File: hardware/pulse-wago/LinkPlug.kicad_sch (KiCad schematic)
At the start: 4 parts, among them J1901 2x05_Horizontal, U1901 THVD24x2

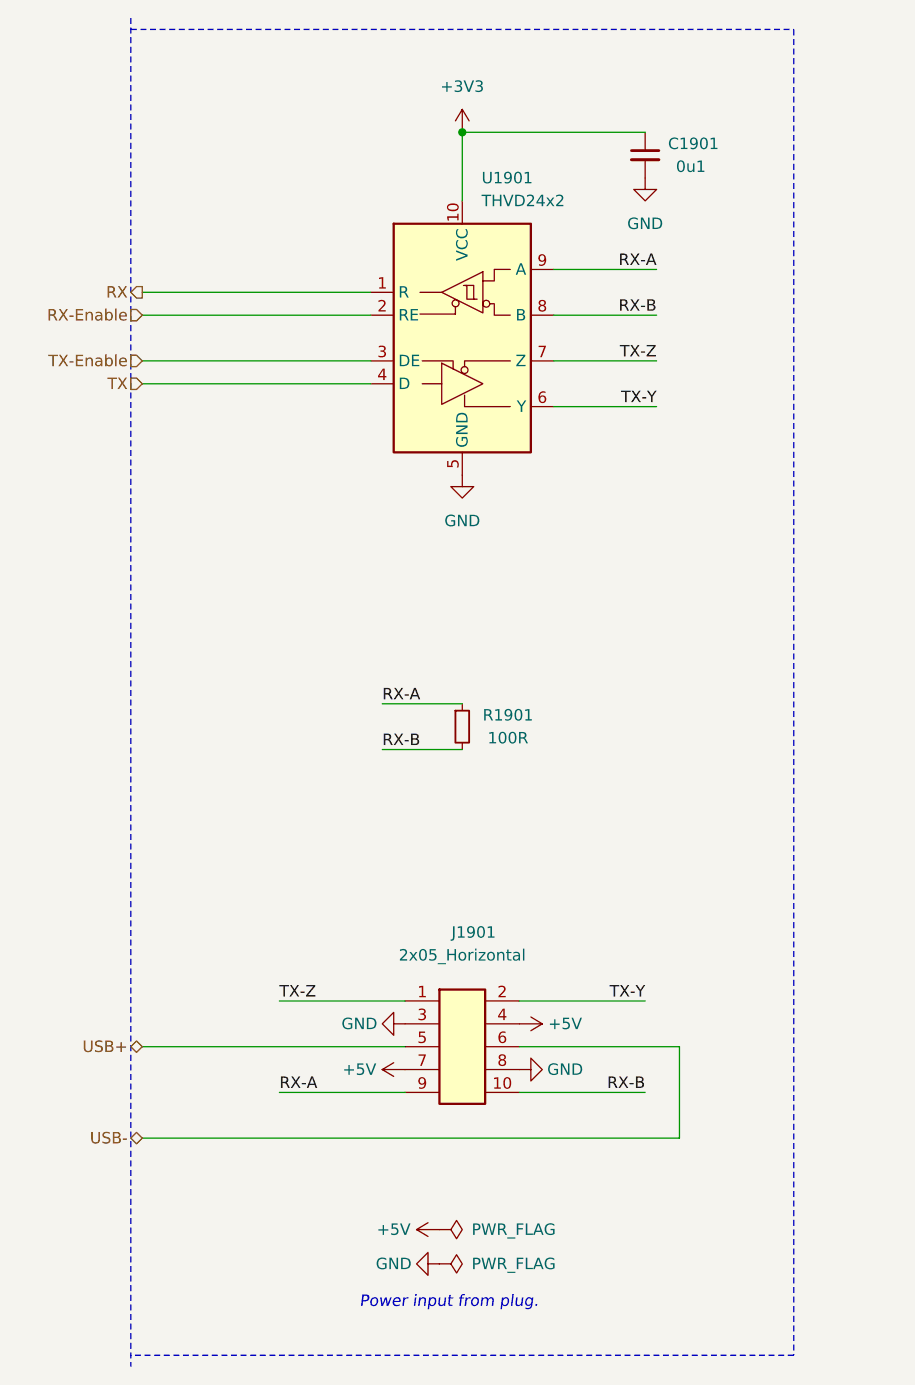
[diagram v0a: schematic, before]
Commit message: Update library
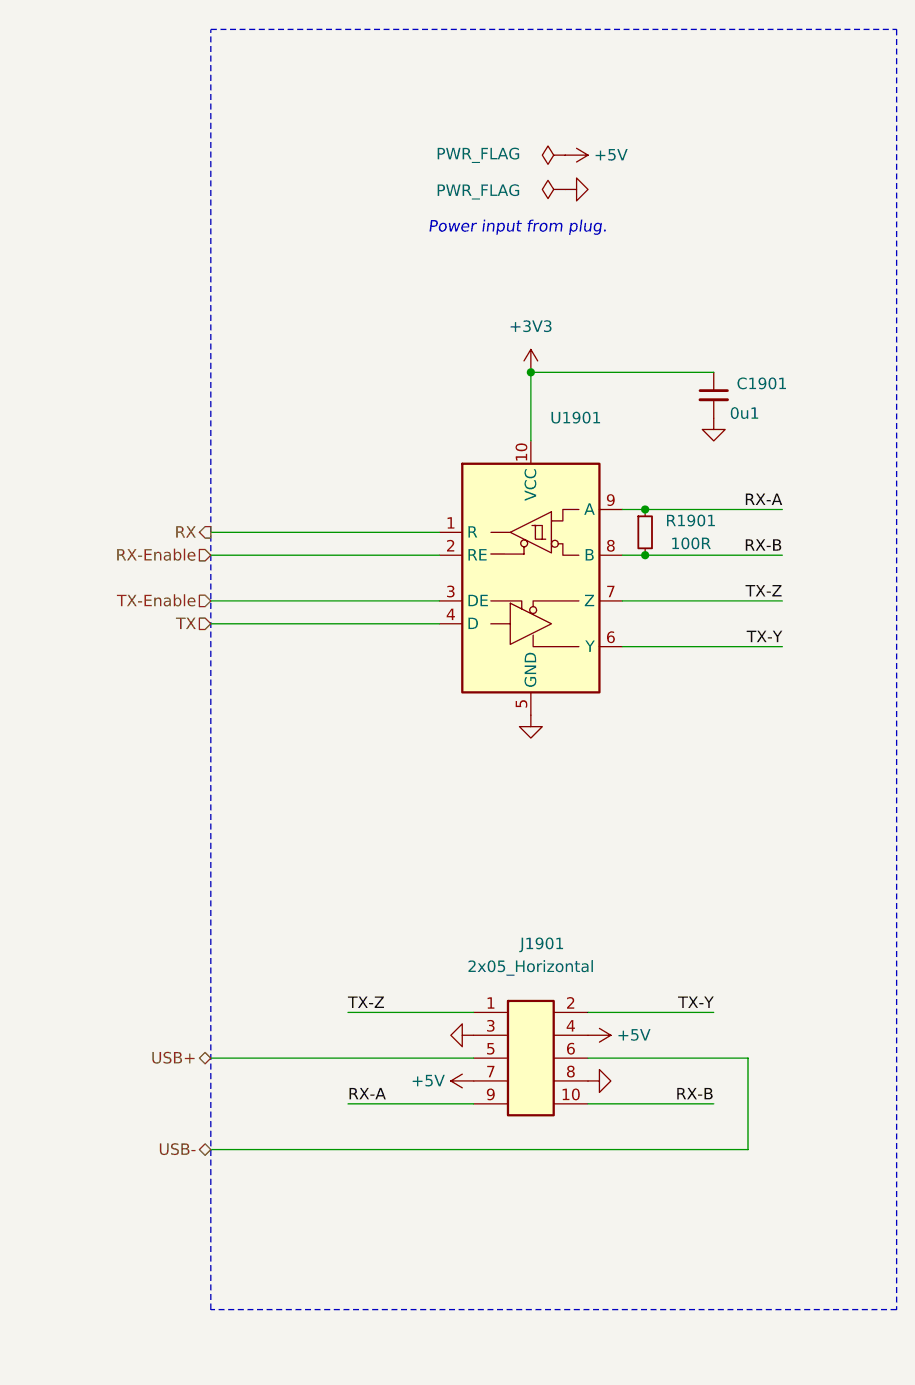
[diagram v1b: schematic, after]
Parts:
- C1901: footprint Capacitor_SMD:C_0603_1608Metric -> V2_Capacitor_SMD:C_0603; symbol Device:C_Small -> V2_Device:C_0603_0u1; Manufacturer (none) -> TDK; Mouser (none) -> 810-CGA3E2X7R1H104MA; Product (none) -> CGA3E2X7R1H104M080AA; Rating (none) -> 50V
- J1901: Manufacturer (none) -> Amphenol FCI; Mouser (none) -> 649-200211120001T4LF; Product (none) -> 20021112-00010T4LF
- R1901: footprint Resistor_SMD:R_0603_1608Metric -> V2_Resistor_SMD:R_0603; symbol Device:R_Small -> V2_Device:R_0603_100R; Manufacturer (none) -> Vishay; Mouser (none) -> 71-CRCW0603100RFKEAH; Product (none) -> CRCW0603100RFKEAHP; Rating (none) -> 330mW
- U1901: value THVD24x2 -> (none)
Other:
- moved on the sheet: C1901, J1901, R1901, U1901

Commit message: Update Library
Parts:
- C1901: symbol V2_Device:C_0603_0u1 -> V2_Capacitor:0603_0u1
- R1901: symbol V2_Device:R_0603_100R -> V2_Resistor:0603_100R
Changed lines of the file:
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@@
 		(on_board yes)
 		(dnp no)
-		(property "Reference" "#PWR01902"
+		(property "Reference" "#PWR1902"
 			(at 176.53 80.01 0)
 			(effects
@@
 			(project "pulse"
 				(path "/6c8448b4-b04d-47e1-934e-e40cbe27a7be/c6db2f80-f80f-4104-8ca1-02f0ab85cfea"
-					(reference "#PWR01902")
+					(reference "#PWR1902")
 					(unit 1)
 				)
@@
 		(on_board yes)
 		(dnp no)
-		(property "Reference" "#FLG01902"
+		(property "Reference" "#FLG1902"
 			(at 160.02 46.355 0)
 			(effects
@@
 			(project "pulse"
 				(path "/6c8448b4-b04d-47e1-934e-e40cbe27a7be/c6db2f80-f80f-4104-8ca1-02f0ab85cfea"
-					(reference "#FLG01902")
+					(reference "#FLG1902")
 					(unit 1)
 				)
@@
 		(on_board yes)
 		(dnp no)
-		(property "Reference" "#FLG01901"
+		(property "Reference" "#FLG1901"
 			(at 160.02 42.545 0)
 			(effects
@@
 			(project "pulse"
 				(path "/6c8448b4-b04d-47e1-934e-e40cbe27a7be/c6db2f80-f80f-4104-8ca1-02f0ab85cfea"
-					(reference "#FLG01901")
+					(reference "#FLG1901")
 					(unit 1)
 				)
@@
 	)
 	(symbol
-		(lib_id "V2_Device:R_0603_100R")
+		(lib_id "V2_Resistor:0603_100R")
 		(at 168.91 86.36 0)
 		(unit 1)
@@
 		(on_board yes)
 		(dnp no)
-		(property "Reference" "#PWR01908"
+		(property "Reference" "#PWR1908"
 			(at 156.21 44.45 0)
 			(effects
@@
 			(project "pulse"
 				(path "/6c8448b4-b04d-47e1-934e-e40cbe27a7be/c6db2f80-f80f-4104-8ca1-02f0ab85cfea"
-					(reference "#PWR01908")
+					(reference "#PWR1908")
 					(unit 1)
 				)
@@
 		(on_board yes)
 		(dnp no)
-		(property "Reference" "#PWR01904"
+		(property "Reference" "#PWR1904"
 			(at 143.51 142.24 0)
 			(effects
@@
 			(project "pulse"
 				(path "/6c8448b4-b04d-47e1-934e-e40cbe27a7be/c6db2f80-f80f-4104-8ca1-02f0ab85cfea"
-					(reference "#PWR01904")
+					(reference "#PWR1904")
 					(unit 1)
 				)
@@
 		(on_board yes)
 		(dnp no)
-		(property "Reference" "#PWR01906"
+		(property "Reference" "#PWR1906"
 			(at 153.67 147.32 0)
 			(effects
@@
 			(project "pulse"
 				(path "/6c8448b4-b04d-47e1-934e-e40cbe27a7be/c6db2f80-f80f-4104-8ca1-02f0ab85cfea"
-					(reference "#PWR01906")
+					(reference "#PWR1906")
 					(unit 1)
 				)
@@
 		(on_board yes)
 		(dnp no)
-		(property "Reference" "#PWR01903"
+		(property "Reference" "#PWR1903"
 			(at 156.21 113.03 0)
 			(effects
@@
 			(project "pulse"
 				(path "/6c8448b4-b04d-47e1-934e-e40cbe27a7be/c6db2f80-f80f-4104-8ca1-02f0ab85cfea"
-					(reference "#PWR01903")
+					(reference "#PWR1903")
 					(unit 1)
 				)
@@
 		(on_board yes)
 		(dnp no)
-		(property "Reference" "#PWR01905"
+		(property "Reference" "#PWR1905"
 			(at 158.75 142.24 0)
 			(effects
@@
 			(project "pulse"
 				(path "/6c8448b4-b04d-47e1-934e-e40cbe27a7be/c6db2f80-f80f-4104-8ca1-02f0ab85cfea"
-					(reference "#PWR01905")
+					(reference "#PWR1905")
 					(unit 1)
 				)
@@
 		(on_board yes)
 		(dnp no)
-		(property "Reference" "#PWR01901"
+		(property "Reference" "#PWR1901"
 			(at 156.21 72.39 0)
 			(effects
@@
 			(project "pulse"
 				(path "/6c8448b4-b04d-47e1-934e-e40cbe27a7be/c6db2f80-f80f-4104-8ca1-02f0ab85cfea"
-					(reference "#PWR01901")
+					(reference "#PWR1901")
 					(unit 1)
 				)
@@
 		(on_board yes)
 		(dnp no)
-		(property "Reference" "#PWR01909"
+		(property "Reference" "#PWR1909"
 			(at 166.37 48.26 0)
 			(effects
@@
 			(project "pulse"
 				(path "/6c8448b4-b04d-47e1-934e-e40cbe27a7be/c6db2f80-f80f-4104-8ca1-02f0ab85cfea"
-					(reference "#PWR01909")
+					(reference "#PWR1909")
 					(unit 1)
 				)
@@
 		(on_board yes)
 		(dnp no)
-		(property "Reference" "#PWR01907"
+		(property "Reference" "#PWR1907"
 			(at 168.91 147.32 0)
 			(effects
@@
 			(project "pulse"
 				(path "/6c8448b4-b04d-47e1-934e-e40cbe27a7be/c6db2f80-f80f-4104-8ca1-02f0ab85cfea"
-					(reference "#PWR01907")
-					(unit 1)
-				)
-			)
-		)
-	)
-	(symbol
-		(lib_id "V2_Device:C_0603_0u1")
+					(reference "#PWR1907")
+					(unit 1)
+				)
+			)
+		)
+	)
+	(symbol
+		(lib_id "V2_Capacitor:0603_0u1")
 		(at 176.53 71.12 0)
 		(unit 1)

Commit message: Update ESD suppressor
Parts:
- U1901: value (none) -> ~
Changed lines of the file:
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@@
 			)
 		)
-		(property "Value" ""
+		(property "Value" "~"
 			(at 158.3533 76.2 0)
 			(effects
